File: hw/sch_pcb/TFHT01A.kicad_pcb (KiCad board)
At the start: 2 copper layers, 30 x 15 mm, 30 parts, among them J1 SM04B-GHS-TB, J2 SM04B-GHS-TB, M1 M3, M2 M3, M3 M3, M4 M3, M5 M3, M6 M3, Q1 BC817, U1 SHT31, U3 MIC5504-3.3YM5

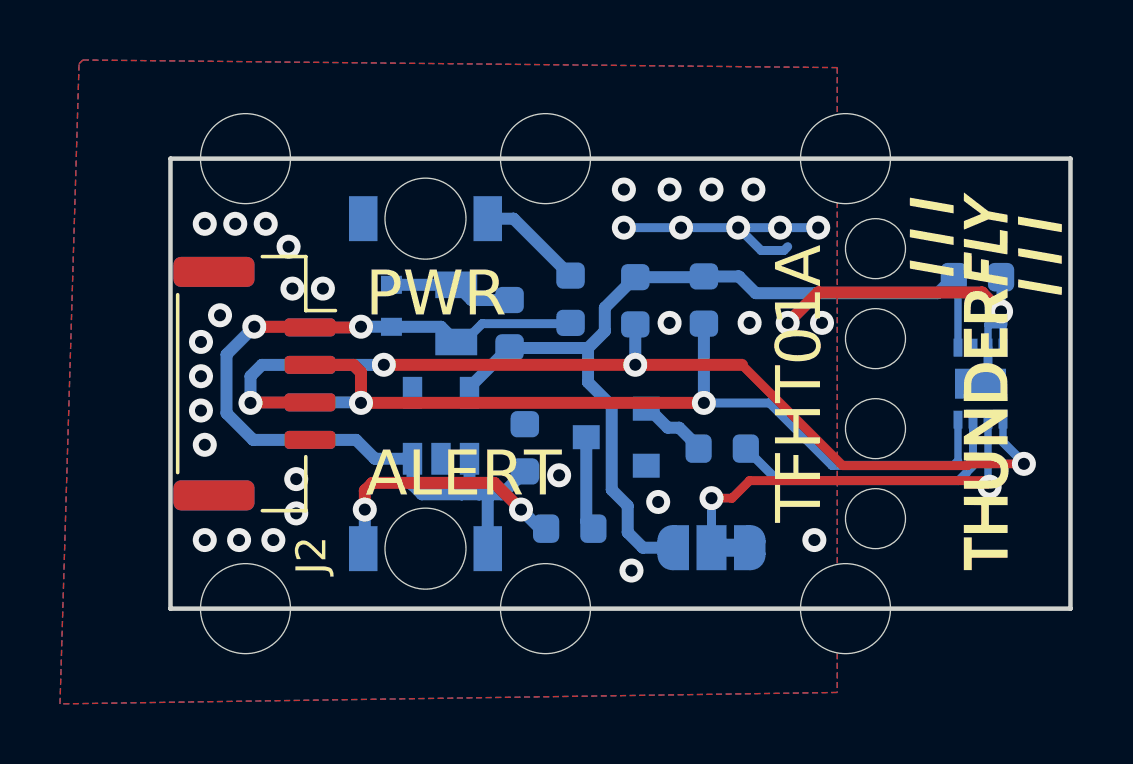
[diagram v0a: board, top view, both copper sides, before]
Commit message: Minor graphics improvement.
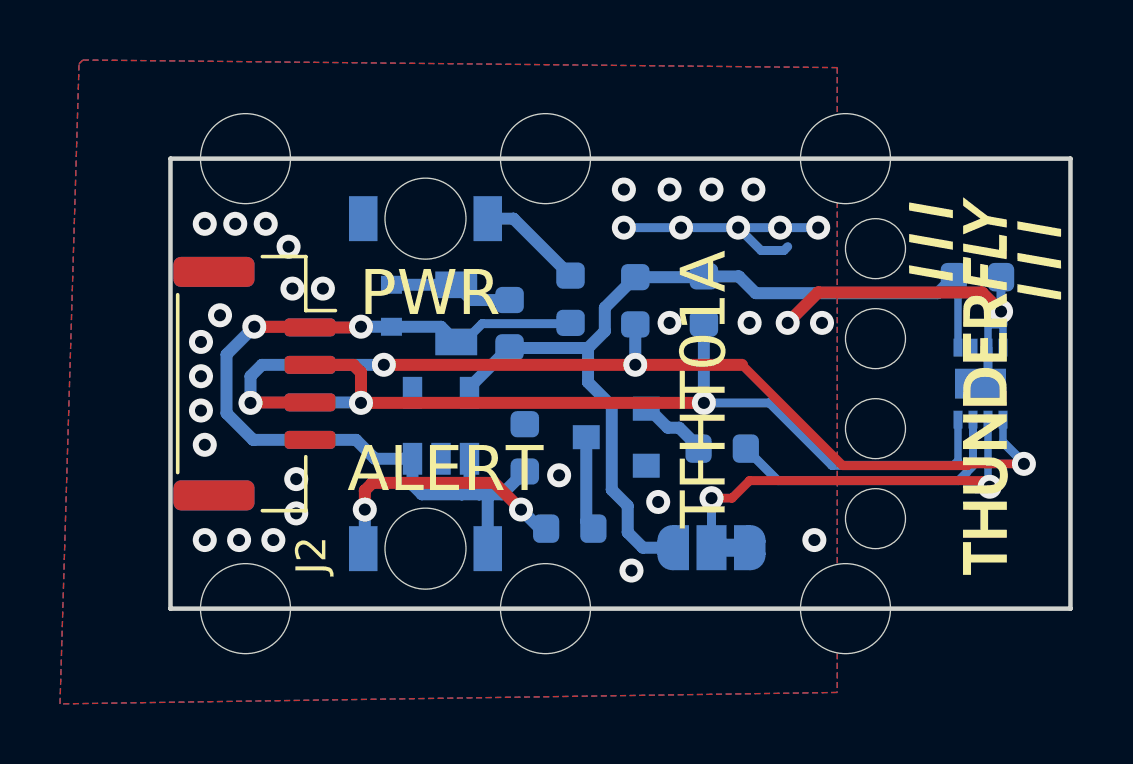
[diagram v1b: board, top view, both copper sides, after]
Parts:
- moved G*** 0.16 mm to (27.2, -7.34)
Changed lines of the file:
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@@
   (net 13 "unconnected-(U3-Pad4)")
   (footprint "MLAB_LOGA:TF 14x6,6" (layer "F.Cu")
-    (at 27.178 -7.5 90)
+    (at 27.1526 -7.3406 90)
     (attr board_only exclude_from_pos_files exclude_from_bom)
     (fp_text reference "G***" (at 0 0 90) (layer "F.SilkS") hide
@@
   )
   (gr_rect (start 0 -15) (end 30 0) (layer "Edge.Cuts") (width 0.15) (fill none))
-  (gr_text "PWR" (at 6.5 -10.5) (layer "F.SilkS")
+  (gr_text "PWR" (at 6.2992 -10.5156) (layer "F.SilkS")
     (effects (font (size 1.5 1.5) (thickness 0.3)) (justify left))
   )
-  (gr_text "TFHT01A" (at 20.955 -7.5 90) (layer "F.SilkS")
+  (gr_text "TFHT01A" (at 17.78 -7.3152 90) (layer "F.SilkS")
     (effects (font (size 1.5 1.5) (thickness 0.3)))
   )
-  (gr_text "ALERT" (at 6.5 -4.5) (layer "F.SilkS")
+  (gr_text "ALERT" (at 5.8928 -4.6482) (layer "F.SilkS")
     (effects (font (size 1.5 1.5) (thickness 0.3)) (justify left))
   )

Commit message: Generating production data
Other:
- rule pad_to_mask_clearance: 0 -> 0.2
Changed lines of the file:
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@@
-(kicad_pcb (version 20210424) (generator pcbnew)
+(kicad_pcb (version 20210228) (generator pcbnew)
   (general
     (thickness 1.6)
@@
       (dielectric_constraints no)
     )
-    (pad_to_mask_clearance 0)
+    (pad_to_mask_clearance 0.2)
     (aux_axis_origin 126.746 136.906)
     (grid_origin 126.746 136.906)
